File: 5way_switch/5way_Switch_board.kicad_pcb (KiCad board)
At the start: 2 copper layers, 35 x 22 mm, 8 parts, among them J1 CONN_01X8, SW1 5way-switch

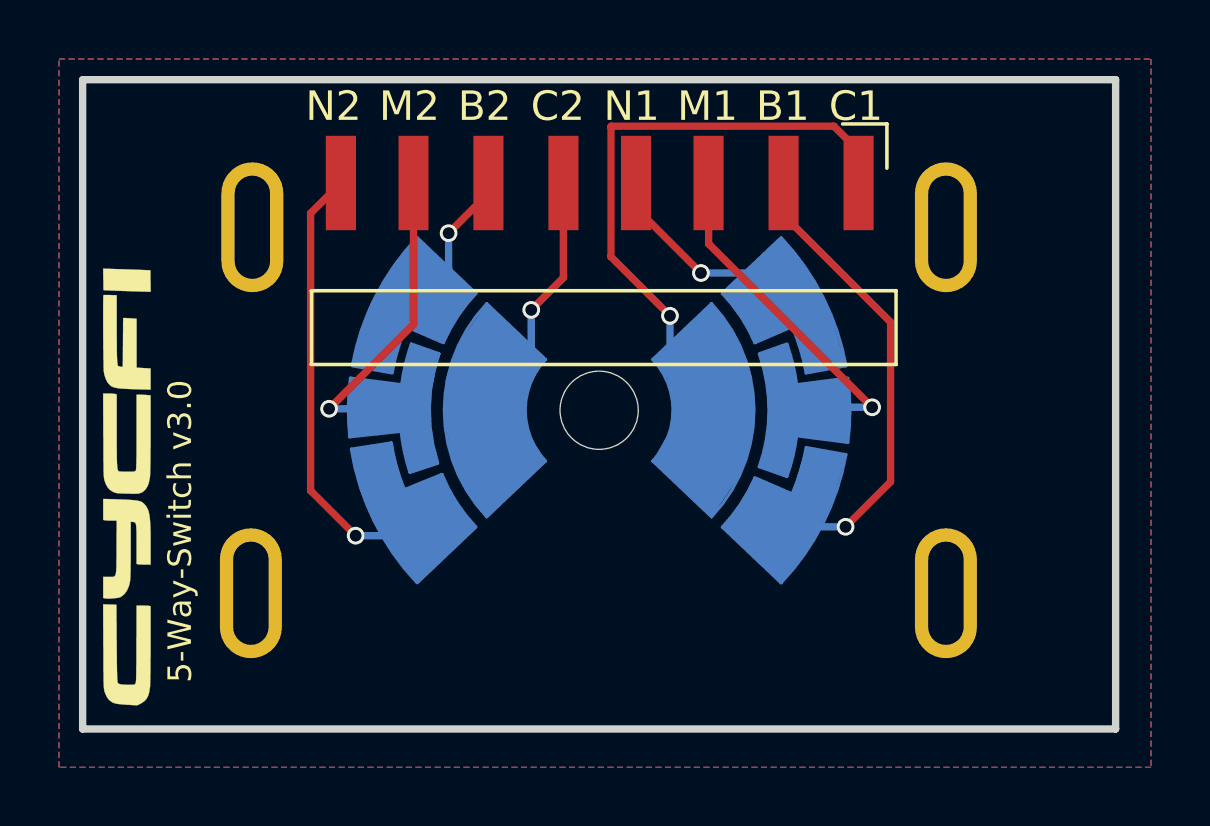
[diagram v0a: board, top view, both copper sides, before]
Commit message: More updates. I think we're good.
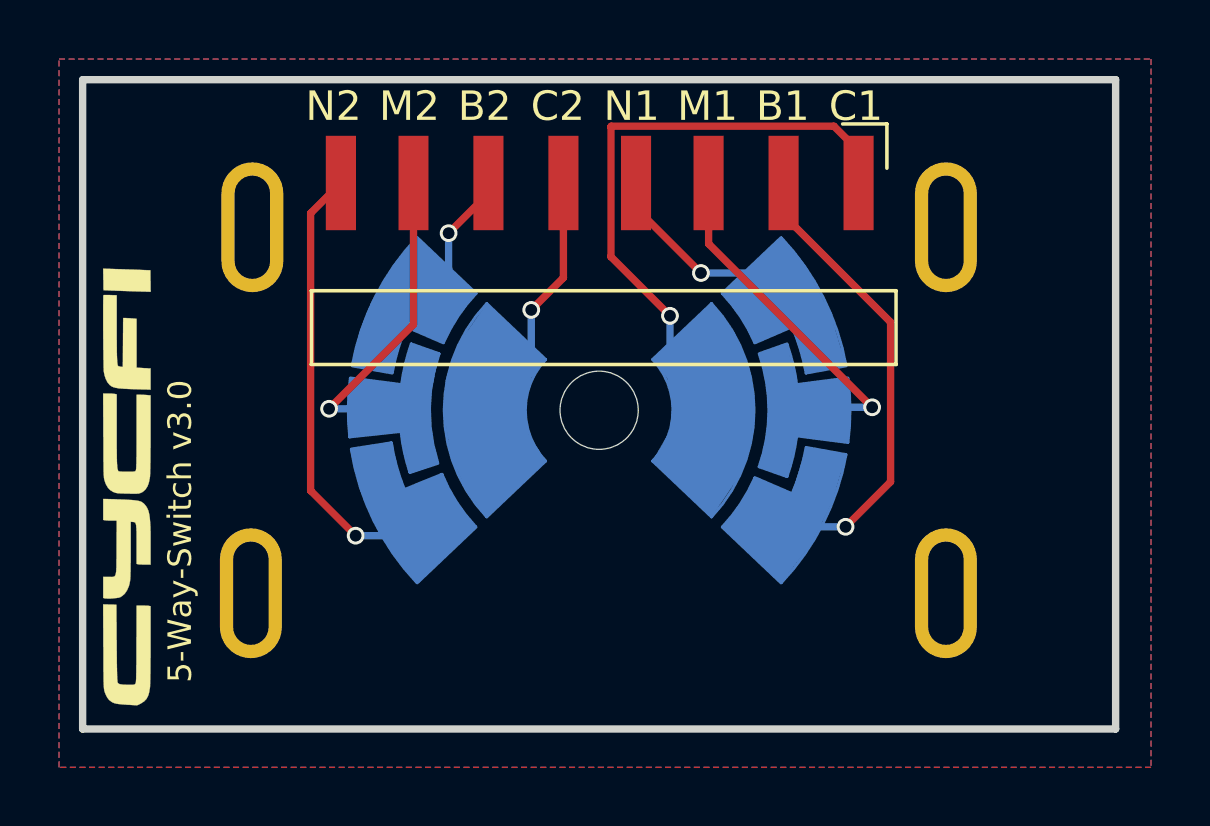
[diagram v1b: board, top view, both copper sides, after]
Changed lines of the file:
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@@
             (gr_line (start -1.012751 -2.540257) (end -2.366089 -2.297148) (width 0.1))
     (gr_arc (start -0.54434 -0.98269) (mid -0.823109 -1.748072) (end -1.012751 -2.540257) (width 0.1))
-    (gr_arc (start -0.18544 2.030115) (mid -1.59044 0.025059) (end -2.366089 -2.297148) (width 0.1))
-    (gr_arc (start 1.829511 0.158474) (mid 1.202376 -0.630683) (end 0.722578 -1.51717) (width 0.1))
+    (gr_arc (start -0.18544 2.030115) (mid -1.587097 0.031686) (end -2.363448 -2.28254) (width 0.1))
+    (gr_arc (start 1.829511 0.158474) (mid 1.205145 -0.626495) (end 0.726574 -1.507958) (width 0.1))
       ))
     (pad "2" smd custom (at -6.9 0 180) (size 1.524 1.524) (layers "B.Cu")
@@
             (xy -1.143 -0.381)
           ) (width 0) (fill yes))
-    (gr_arc (start 1.468521 1.887188) (mid 1.150193 -0.015059) (end 1.478475 -1.915614) (width 0.1))
+    (gr_arc (start 1.468521 1.887188) (mid 1.150193 -0.015059) (end 1.478475 -1.915613) (width 0.1))
             (gr_line (start 1.478475 -1.915614) (end 0.535602 -2.248764) (width 0.1))
             (gr_line (start 0.535602 2.248763) (end 1.478475 1.915613) (width 0.1))
-    (gr_arc (start 0.210716 -0.903391) (mid 0.338493 -1.584449) (end 0.535602 -2.248764) (width 0.1))
+    (gr_arc (start 0.210716 -0.903391) (mid 0.33849 -1.584436) (end 0.535593 -2.248739) (width 0.1))
             (gr_line (start 0.206103 -0.868475) (end -1.529351 -1.093636) (width 0.1))
-    (gr_arc (start -1.533117 1.064237) (mid -1.60006 -0.01482) (end -1.529351 -1.093636) (width 0.1))
+    (gr_arc (start -1.533117 1.064237) (mid -1.60007 -0.007414) (end -1.531246 -1.078946) (width 0.1))
             (gr_line (start -1.529351 1.093635) (end 0.206103 0.868475) (width 0.1))
-    (gr_arc (start 0.527809 2.226602) (mid 0.331665 1.555898) (end 0.206103 0.868475) (width 0.1))
+    (gr_arc (start 0.527809 2.226602) (mid 0.333021 1.561612) (end 0.207621 0.880122) (width 0.1))
             (gr_poly (pts
             (xy 1.478475 1.915613)
@@
             (gr_line (start 1.929527 -0.158491) (end -0.065048 -2.051683) (width 0.1))
             (gr_line (start -2.266089 2.297148) (end -0.912751 2.540256) (width 0.1))
-    (gr_arc (start -0.90831 2.515788) (mid -0.717714 1.730219) (end -0.439415 0.971275) (width 0.1))
-    (gr_arc (start -2.263448 2.282536) (mid -1.480395 -0.044929) (end -0.065048 -2.051683) (width 0.1))
-    (gr_arc (start 0.830582 1.498761) (mid 1.307924 0.622304) (end 1.929527 -0.158491) (width 0.1))
+    (gr_arc (start -0.90831 2.515788) (mid -0.719516 1.736164) (end -0.444337 0.982684) (width 0.1))
+    (gr_arc (start -2.263448 2.282536) (mid -1.483748 -0.03831) (end -0.075253 -2.040908) (width 0.1))
+    (gr_arc (start 0.830582 1.498761) (mid 1.305154 0.626486) (end 1.922628 -0.151208) (width 0.1))
       ))
     (pad "4" smd custom (at -3.8 0 180) (size 1.524 1.524) (layers "B.Cu")
@@
             (gr_line (start 1.139203 2.797621) (end 2.497646 2.584881) (width 0.1))
             (gr_line (start 0.265047 -1.951683) (end -1.729527 -0.058491) (width 0.1))
-    (gr_arc (start 0.285433 -1.930128) (mid 1.732955 0.160094) (end 2.497646 2.584881) (width 0.1))
-    (gr_arc (start 0.712637 1.246919) (mid 0.969948 2.010159) (end 1.139203 2.797621) (width 0.1))
+    (gr_arc (start 0.285433 -1.930128) (mid 1.729688 0.153434) (end 2.495337 2.570226) (width 0.1))
+    (gr_arc (start 0.712637 1.246919) (mid 0.969946 2.010153) (end 1.139201 2.797609) (width 0.1))
     (gr_arc (start -1.715715 -0.043877) (mid -1.063286 0.790947) (end -0.574737 1.731114) (width 0.1))
       ))
@@
           ) (width 0) (fill yes))
             (gr_line (start -0.606104 0.768475) (end 1.129351 0.993635) (width 0.1))
-    (gr_arc (start -0.607622 0.780122) (mid -0.735748 1.473037) (end -0.935602 2.148763) (width 0.1))
+    (gr_arc (start -0.607622 0.780122) (mid -0.735747 1.473031) (end -0.935598 2.148752) (width 0.1))
             (gr_line (start -1.878476 1.815613) (end -0.935602 2.148763) (width 0.1))
-    (gr_arc (start -1.82922 -1.870054) (mid -1.550421 -0.023165) (end -1.878476 1.815613) (width 0.1))
+    (gr_arc (start -1.82922 -1.870054) (mid -1.550356 -0.028181) (end -1.875141 1.806152) (width 0.1))
             (gr_line (start -0.888744 -2.211467) (end -1.83856 -1.898657) (width 0.1))
-    (gr_arc (start 1.151731 -1.004571) (mid 1.199461 -0.004808) (end 1.129351 0.993635) (width 0.1))
+    (gr_arc (start 1.151731 -1.004571) (mid 1.199541 -0.012223) (end 1.131246 0.978926) (width 0.1))
             (gr_line (start 1.151729 -1.004589) (end -0.588333 -0.81835) (width 0.1))
-    (gr_arc (start -0.881411 -2.189057) (mid -0.699254 -1.511319) (end -0.588333 -0.81835) (width 0.1))
+    (gr_arc (start -0.881411 -2.189057) (mid -0.70049 -1.517087) (end -0.589601 -0.83008) (width 0.1))
             (gr_poly (pts
             (xy -0.606104 0.768475)
@@
             (gr_line (start 0.539414 -1.071276) (end -0.722578 -1.61717) (width 0.1))
             (gr_line (start 2.366088 -2.397148) (end 1.01275 -2.640257) (width 0.1))
-    (gr_arc (start -0.734602 -1.589582) (mid -1.210695 -0.71813) (end -1.829527 0.058491) (width 0.1))
-    (gr_arc (start 2.363447 -2.382536) (mid 1.580394 -0.055071) (end 0.165047 1.951683) (width 0.1))
-    (gr_arc (start 1.008309 -2.615789) (mid 0.817713 -1.83022) (end 0.539414 -1.071276) (width 0.1))
+    (gr_arc (start -0.734602 -1.589582) (mid -1.210693 -0.718132) (end -1.829523 0.058487) (width 0.1))
+    (gr_arc (start 2.363447 -2.382536) (mid 1.583747 -0.06169) (end 0.175252 1.940908) (width 0.1))
+    (gr_arc (start 1.008309 -2.615789) (mid 0.819515 -1.836165) (end 0.544336 -1.082685) (width 0.1))
       ))
     (pad "8" smd custom (at 3.7 -0.1 180) (size 1.524 1.524) (layers "B.Cu")
